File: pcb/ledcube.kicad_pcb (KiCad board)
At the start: 2 copper layers, 194.5 x 8 mm, 24 parts

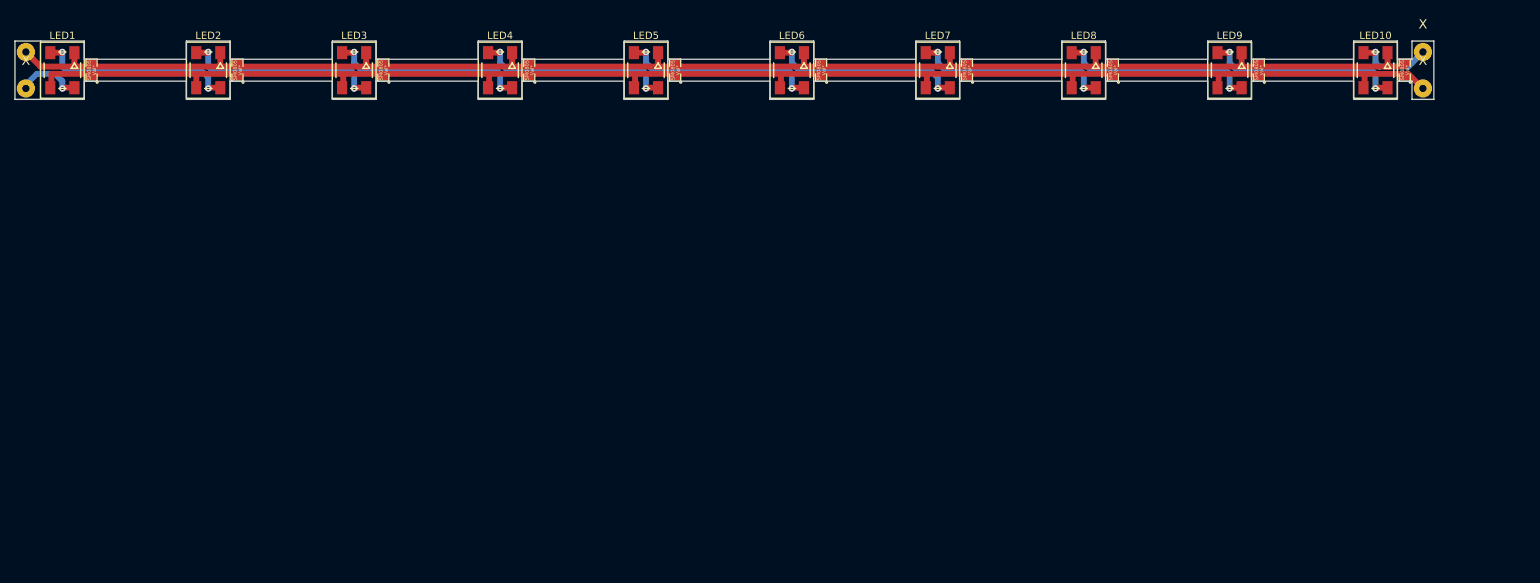
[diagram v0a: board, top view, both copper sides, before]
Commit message: Schematic, components placed.
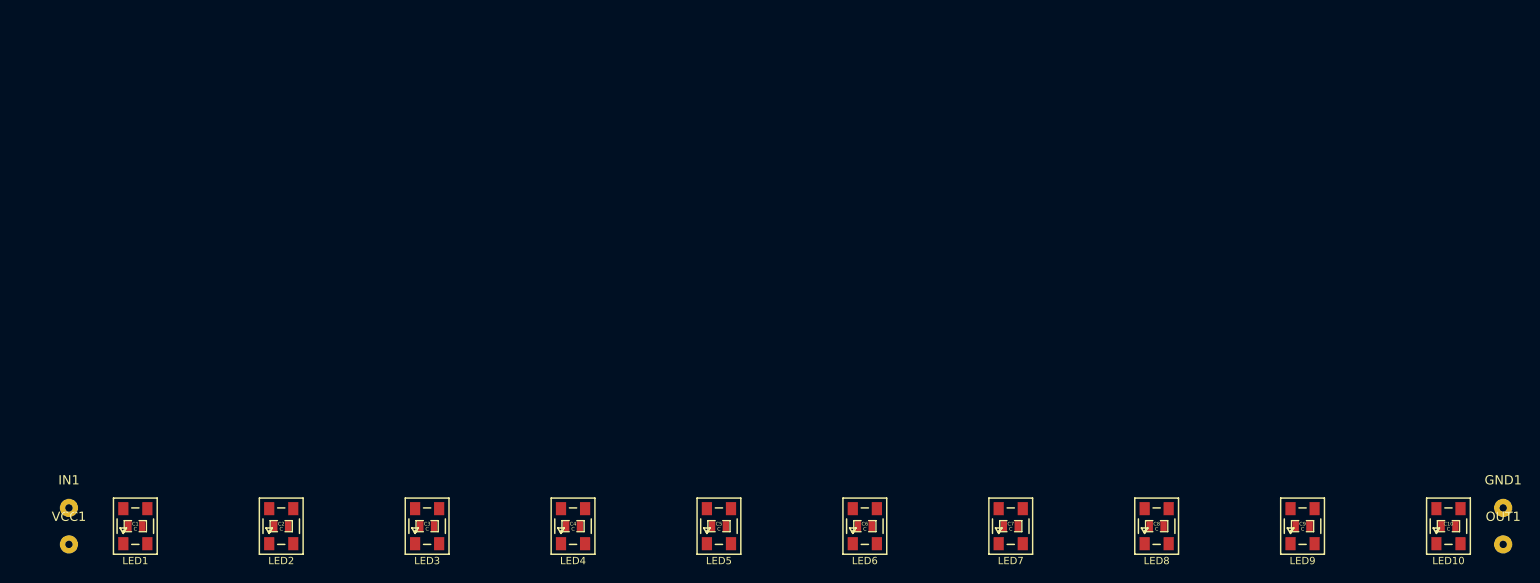
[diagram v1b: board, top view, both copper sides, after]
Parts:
- removed SM0805 (x10): Val*, SMD_Packages:SM0805
- removed X (x4): SolderWirePad_single_1mmDrill, Wire_Pads:SolderWirePad_single_1mmDrill
- added C1: C, SMD_Packages:SMD-0805, F.Cu at (60.0, 102.5)
- added C10: C, SMD_Packages:SMD-0805, F.Cu at (240.0, 102.5)
- added C2: C, SMD_Packages:SMD-0805, F.Cu at (80.0, 102.5)
- added C3: C, SMD_Packages:SMD-0805, F.Cu at (100.0, 102.5)
- added C4: C, SMD_Packages:SMD-0805, F.Cu at (120.0, 102.5)
- added C5: C, SMD_Packages:SMD-0805, F.Cu at (140.0, 102.5)
- added C6: C, SMD_Packages:SMD-0805, F.Cu at (160.0, 102.5)
- added C7: C, SMD_Packages:SMD-0805, F.Cu at (180.0, 102.5)
- added C8: C, SMD_Packages:SMD-0805, F.Cu at (200.0, 102.5)
- added C9: C, SMD_Packages:SMD-0805, F.Cu at (220.0, 102.5)
- added GND1: CONN_1, Wire_Pads:SolderWirePad_single_1mmDrill, F.Cu at (247.5, 100.0)
- added IN1: CONN_1, Wire_Pads:SolderWirePad_single_1mmDrill, F.Cu at (50.9, 100.0)
- added OUT1: CONN_1, Wire_Pads:SolderWirePad_single_1mmDrill, F.Cu at (247.5, 105.0)
- added VCC1: CONN_1, Wire_Pads:SolderWirePad_single_1mmDrill, F.Cu at (50.9, 105.0)
- LED1, LED10, LED2, LED3, LED4, LED5, LED6, LED7, LED8, LED9: value VAL** -> WS2812B
- moved LED1 63.3 mm to (60.0, 102.5), turned to 180 degrees
- moved LED10 63.3 mm to (240.0, 102.5), turned to 180 degrees
- moved LED2 63.3 mm to (80.0, 102.5), turned to 180 degrees
- moved LED3 63.3 mm to (100.0, 102.5), turned to 180 degrees
- moved LED4 63.3 mm to (120.0, 102.5), turned to 180 degrees
- moved LED5 63.3 mm to (140.0, 102.5), turned to 180 degrees
- moved LED6 63.3 mm to (160.0, 102.5), turned to 180 degrees
- moved LED7 63.3 mm to (180.0, 102.5), turned to 180 degrees
- moved LED8 63.3 mm to (200.0, 102.5), turned to 180 degrees
- moved LED9 63.3 mm to (220.0, 102.5), turned to 180 degrees
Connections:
- LED1 pad 1: (no net) -> Net-(C1-Pad1)
- LED1 pad 2: (no net) -> Net-(LED1-Pad2)
- LED1 pad 3: (no net) -> Net-(C1-Pad2)
- LED1 pad 4: (no net) -> Net-(IN1-Pad1)
- LED10 pad 1: (no net) -> Net-(C1-Pad1)
- LED10 pad 2: (no net) -> Net-(LED10-Pad2)
- LED10 pad 3: (no net) -> Net-(C1-Pad2)
- LED10 pad 4: (no net) -> Net-(LED10-Pad4)
- LED2 pad 1: (no net) -> Net-(C1-Pad1)
- LED2 pad 2: (no net) -> Net-(LED2-Pad2)
- LED2 pad 3: (no net) -> Net-(C1-Pad2)
- LED2 pad 4: (no net) -> Net-(LED1-Pad2)
- LED3 pad 1: (no net) -> Net-(C1-Pad1)
- LED3 pad 2: (no net) -> Net-(LED3-Pad2)
- LED3 pad 3: (no net) -> Net-(C1-Pad2)
- LED3 pad 4: (no net) -> Net-(LED2-Pad2)
- LED4 pad 1: (no net) -> Net-(C1-Pad1)
- LED4 pad 2: (no net) -> Net-(LED4-Pad2)
- LED4 pad 3: (no net) -> Net-(C1-Pad2)
- LED4 pad 4: (no net) -> Net-(LED3-Pad2)
- LED5 pad 1: (no net) -> Net-(C1-Pad1)
- LED5 pad 2: (no net) -> Net-(LED5-Pad2)
- LED5 pad 3: (no net) -> Net-(C1-Pad2)
- LED5 pad 4: (no net) -> Net-(LED4-Pad2)
- LED6 pad 1: (no net) -> Net-(C1-Pad1)
- LED6 pad 2: (no net) -> Net-(LED6-Pad2)
- LED6 pad 3: (no net) -> Net-(C1-Pad2)
- LED6 pad 4: (no net) -> Net-(LED5-Pad2)
- LED7 pad 1: (no net) -> Net-(C1-Pad1)
- LED7 pad 2: (no net) -> Net-(LED7-Pad2)
- LED7 pad 3: (no net) -> Net-(C1-Pad2)
- LED7 pad 4: (no net) -> Net-(LED6-Pad2)
- LED8 pad 1: (no net) -> Net-(C1-Pad1)
- LED8 pad 2: (no net) -> Net-(LED8-Pad2)
- LED8 pad 3: (no net) -> Net-(C1-Pad2)
- LED8 pad 4: (no net) -> Net-(LED7-Pad2)
- LED9 pad 1: (no net) -> Net-(C1-Pad1)
- LED9 pad 2: (no net) -> Net-(LED10-Pad4)
- LED9 pad 3: (no net) -> Net-(C1-Pad2)
- LED9 pad 4: (no net) -> Net-(LED8-Pad2)
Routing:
- net (no net): track 686.7 -> 0.00 mm, vias 20 -> 0
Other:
- board outline removed
